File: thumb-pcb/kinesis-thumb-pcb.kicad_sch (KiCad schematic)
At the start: 25 parts, among them J1 Conn_01x10

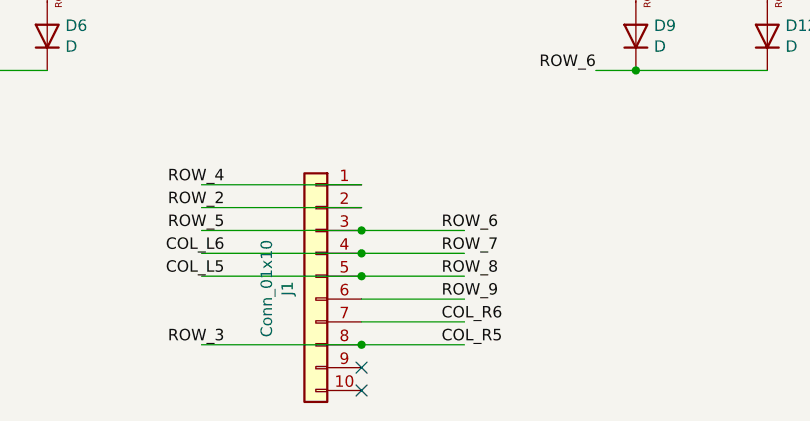
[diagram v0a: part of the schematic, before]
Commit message: Update files and readme
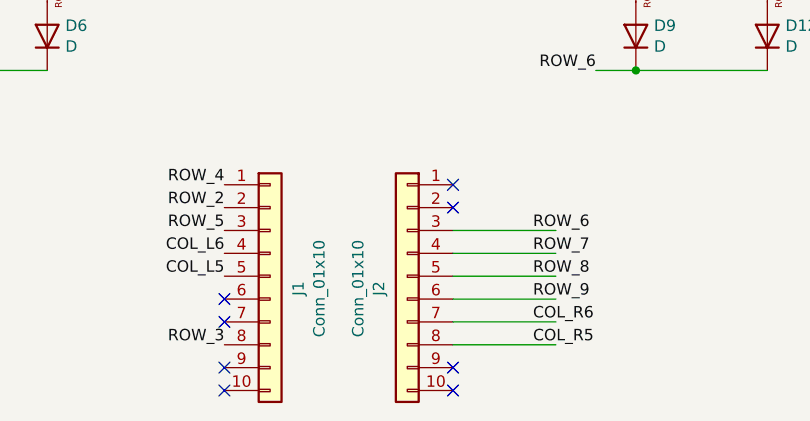
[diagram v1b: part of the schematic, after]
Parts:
- added J2: Conn_01x10, Pin_Headers:Pin_Header_Straight_1x10_Pitch2.54mm, symbol kicad_port-rescue:Conn_01x10-Connector_Generic
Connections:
- net COL_L5: no longer D10.1 (K), D8.1 (K)
- net COL_L6: no longer D11.1 (K)
- net COL_R5: now also J2.8 (Pin_8); no longer D3.1 (K), D5.1 (K), J1.8 (Pin_8)
- net COL_R6: now also J2.7 (Pin_7); no longer J1.7 (Pin_7)
- net ROW_5: no longer D12.1 (K), D9.1 (K)
- net ROW_9: now also J2.6 (Pin_6); no longer J1.6 (Pin_6)
- new net ROW_3: D3.1 (K), D5.1 (K), J1.8 (Pin_8)
- new net ROW_6: D12.1 (K), D9.1 (K), J2.3 (Pin_3)
- new net ROW_7: D11.1 (K), J2.4 (Pin_4)
- new net ROW_8: D10.1 (K), D8.1 (K), J2.5 (Pin_5)
- no-connect marks 2 -> 8
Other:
- company: Dmitriy Nosachev -> dcpedit
- title: Kinesis80 thumb cluster PCB -> PillzMod thumb cluster PCB
- moved on the sheet: J1
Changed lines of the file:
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@@
   (paper "A4")
   (title_block
-    (title "Kinesis80 thumb cluster PCB")
-    (date "2022-03-15")
-    (rev "1.3")
-    (company "Dmitriy Nosachev")
+    (title "PillzMod thumb cluster PCB")
+    (date "2024-03-13")
+    (rev "1")
+    (company "dcpedit")
   )
   (junction (at 55.88 34.925) (diameter 0) (color 0 0 0 0)
@@
   (junction (at 36.195 86.995) (diameter 0) (color 0 0 0 0)
   )
-  (junction (at 85.725 127) (diameter 0) (color 0 0 0 0)
-  )
   (junction (at 41.275 34.925) (diameter 0) (color 0 0 0 0)
   )
@@
   (junction (at 121.285 34.925) (diameter 0) (color 0 0 0 0)
   )
-  (junction (at 85.725 129.54) (diameter 0) (color 0 0 0 0)
-  )
-  (junction (at 85.725 137.16) (diameter 0) (color 0 0 0 0)
-  )
   (junction (at 121.285 54.61) (diameter 0) (color 0 0 0 0)
   )
@@
   (junction (at 55.88 74.295) (diameter 0) (color 0 0 0 0)
   )
-  (junction (at 85.725 124.46) (diameter 0) (color 0 0 0 0)
-  )
   (junction (at 116.205 106.68) (diameter 0) (color 0 0 0 0)
   )
-  (no_connect (at 85.725 142.24))
-  (no_connect (at 85.725 139.7))
-  (wire (pts (xy 67.945 121.92) (xy 85.725 121.92))
-    (stroke (width 0) (type default))
-  )
+  (no_connect (at 95.885 139.7))
+  (no_connect (at 70.485 139.7))
+  (no_connect (at 70.485 142.24))
+  (no_connect (at 95.885 119.38))
+  (no_connect (at 70.485 132.08))
+  (no_connect (at 95.885 142.24))
+  (no_connect (at 95.885 121.92))
+  (no_connect (at 70.485 134.62))
   (wire (pts (xy 31.75 86.995) (xy 36.195 86.995))
     (stroke (width 0) (type default))
@@
     (stroke (width 0) (type default))
   )
-  (wire (pts (xy 67.945 119.38) (xy 85.725 119.38))
-    (stroke (width 0) (type default))
-  )
   (wire (pts (xy 31.75 47.625) (xy 36.195 47.625))
     (stroke (width 0) (type default))
@@
     (stroke (width 0) (type default))
   )
-  (wire (pts (xy 85.725 129.54) (xy 97.155 129.54))
+  (wire (pts (xy 95.885 129.54) (xy 107.315 129.54))
     (stroke (width 0) (type default))
   )
@@
     (stroke (width 0) (type default))
   )
-  (wire (pts (xy 67.945 124.46) (xy 85.725 124.46))
-    (stroke (width 0) (type default))
-  )
   (wire (pts (xy 135.89 54.61) (xy 135.89 74.295))
     (stroke (width 0) (type default))
   )
-  (wire (pts (xy 67.945 129.54) (xy 85.725 129.54))
-    (stroke (width 0) (type default))
-  )
-  (wire (pts (xy 85.725 127) (xy 97.155 127))
+  (wire (pts (xy 95.885 127) (xy 107.315 127))
     (stroke (width 0) (type default))
   )
@@
     (stroke (width 0) (type default))
   )
-  (wire (pts (xy 85.725 132.08) (xy 97.155 132.08))
-    (stroke (width 0) (type default))
-  )
-  (wire (pts (xy 67.945 127) (xy 85.725 127))
+  (wire (pts (xy 95.885 132.08) (xy 107.315 132.08))
     (stroke (width 0) (type default))
   )
@@
     (stroke (width 0) (type default))
   )
-  (wire (pts (xy 67.945 137.16) (xy 85.725 137.16))
-    (stroke (width 0) (type default))
-  )
-  (wire (pts (xy 85.725 124.46) (xy 97.155 124.46))
+  (wire (pts (xy 95.885 124.46) (xy 107.315 124.46))
     (stroke (width 0) (type default))
   )
@@
     (stroke (width 0) (type default))
   )
-  (wire (pts (xy 85.725 137.16) (xy 97.155 137.16))
+  (wire (pts (xy 95.885 137.16) (xy 107.315 137.16))
     (stroke (width 0) (type default))
   )
@@
     (stroke (width 0) (type default))
   )
-  (wire (pts (xy 85.725 134.62) (xy 97.155 134.62))
+  (wire (pts (xy 95.885 134.62) (xy 107.315 134.62))
     (stroke (width 0) (type default))
   )
@@
     (effects (font (size 1.27 1.27)) (justify right bottom))
   )
-  (label "COL_R6" (at 94.615 134.62 0) (fields_autoplaced)
+  (label "COL_R6" (at 104.775 134.62 0) (fields_autoplaced)
     (effects (font (size 1.27 1.27)) (justify left bottom))
   )
-  (label "ROW_6" (at 94.615 124.46 0) (fields_autoplaced)
+  (label "ROW_6" (at 104.775 124.46 0) (fields_autoplaced)
     (effects (font (size 1.27 1.27)) (justify left bottom))
   )
-  (label "ROW_9" (at 94.615 132.08 0) (fields_autoplaced)
+  (label "ROW_9" (at 104.775 132.08 0) (fields_autoplaced)
     (effects (font (size 1.27 1.27)) (justify left bottom))
   )
@@
     (effects (font (size 1.27 1.27)) (justify right bottom))
   )
-  (label "ROW_7" (at 94.615 127 0) (fields_autoplaced)
+  (label "ROW_7" (at 104.775 127 0) (fields_autoplaced)
     (effects (font (size 1.27 1.27)) (justify left bottom))
   )
@@
     (effects (font (size 1.27 1.27)) (justify right bottom))
   )
-  (label "ROW_8" (at 94.615 129.54 0) (fields_autoplaced)
+  (label "ROW_8" (at 104.775 129.54 0) (fields_autoplaced)
     (effects (font (size 1.27 1.27)) (justify left bottom))
   )
-  (label "COL_R5" (at 94.615 137.16 0) (fields_autoplaced)
+  (label "COL_R5" (at 104.775 137.16 0) (fields_autoplaced)
     (effects (font (size 1.27 1.27)) (justify left bottom))
   )
@@
     )
   )
+  (symbol (lib_id "kicad_port-rescue:Conn_01x10-Connector_Generic") (at 90.805 129.54 0) (mirror y) (unit 1)
+    (in_bom yes) (on_board yes) (dnp no)
+    (property "Reference" "J2" (at 87.6554 130.9116 90)
+      (effects (font (size 1.27 1.27)))
+    )
+    (property "Value" "Conn_01x10" (at 85.344 130.9116 90)
+      (effects (font (size 1.27 1.27)))
+    )
+    (property "Footprint" "Pin_Headers:Pin_Header_Straight_1x10_Pitch2.54mm" (at 90.805 129.54 0)
+      (effects (font (size 1.27 1.27)) hide)
+    )
+    (property "Datasheet" "~" (at 90.805 129.54 0)
+      (effects (font (size 1.27 1.27)) hide)
+    )
+    (pin "1")
+    (pin "10")
+    (pin "2")
+    (pin "3")
+    (pin "4")
+    (pin "5")
+    (pin "6")
+    (pin "7")
+    (pin "8")
+    (pin "9")
+    (instances
+      (project "kinesis-thumb-pcb"
+        (path "/c801d42e-dd94-493e-bd2f-6c3ddad43f55"
+          (reference "J2") (unit 1)
+        )
+      )
+    )
+  )
   (symbol (lib_id "MX_Alps_Hybrid:MX-NoLED") (at 52.07 36.195 0) (unit 1)
     (in_bom yes) (on_board yes) (dnp no)
@@
     )
   )
-  (symbol (lib_id "kicad_port-rescue:Conn_01x10-Connector_Generic") (at 80.645 129.54 0) (mirror y) (unit 1)
-    (in_bom yes) (on_board yes) (dnp no)
-    (property "Reference" "J1" (at 77.4954 130.9116 90)
+  (symbol (lib_id "kicad_port-rescue:Conn_01x10-Connector_Generic") (at 75.565 129.54 0) (unit 1)
+    (in_bom yes) (on_board yes) (dnp no)
+    (property "Reference" "J1" (at 78.7146 130.9116 90)
       (effects (font (size 1.27 1.27)))
     )
-    (property "Value" "Conn_01x10" (at 75.184 130.9116 90)
+    (property "Value" "Conn_01x10" (at 81.026 130.9116 90)
       (effects (font (size 1.27 1.27)))
     )
-    (property "Footprint" "Pin_Headers:Pin_Header_Straight_1x10_Pitch2.54mm" (at 80.645 129.54 0)
-      (effects (font (size 1.27 1.27)) hide)
-    )
-    (property "Datasheet" "~" (at 80.645 129.54 0)
-      (effects (font (size 1.27 1.27)) hide)
-    )
+    (property "Footprint" "Pin_Headers:Pin_Header_Straight_1x10_Pitch2.54mm" (at 75.565 129.54 0)
+      (effects (font (size 1.27 1.27)) hide)
+    )
+    (property "Datasheet" "~" (at 75.565 129.54 0)
+      (effects (font (size 1.27 1.27)) hide)
+    )
